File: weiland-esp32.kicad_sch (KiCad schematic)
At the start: 19 parts, among them J1 Conn_01x04_Pin, J2 Conn_01x05_Pin, J5 Conn_02x03_Odd_Even, U1 ESP32-WROOM-32E(8MB), U2 AMS1117-3.3_C347222, U3 GR6205-SOP-8, U4 MAX98357AEWL_T

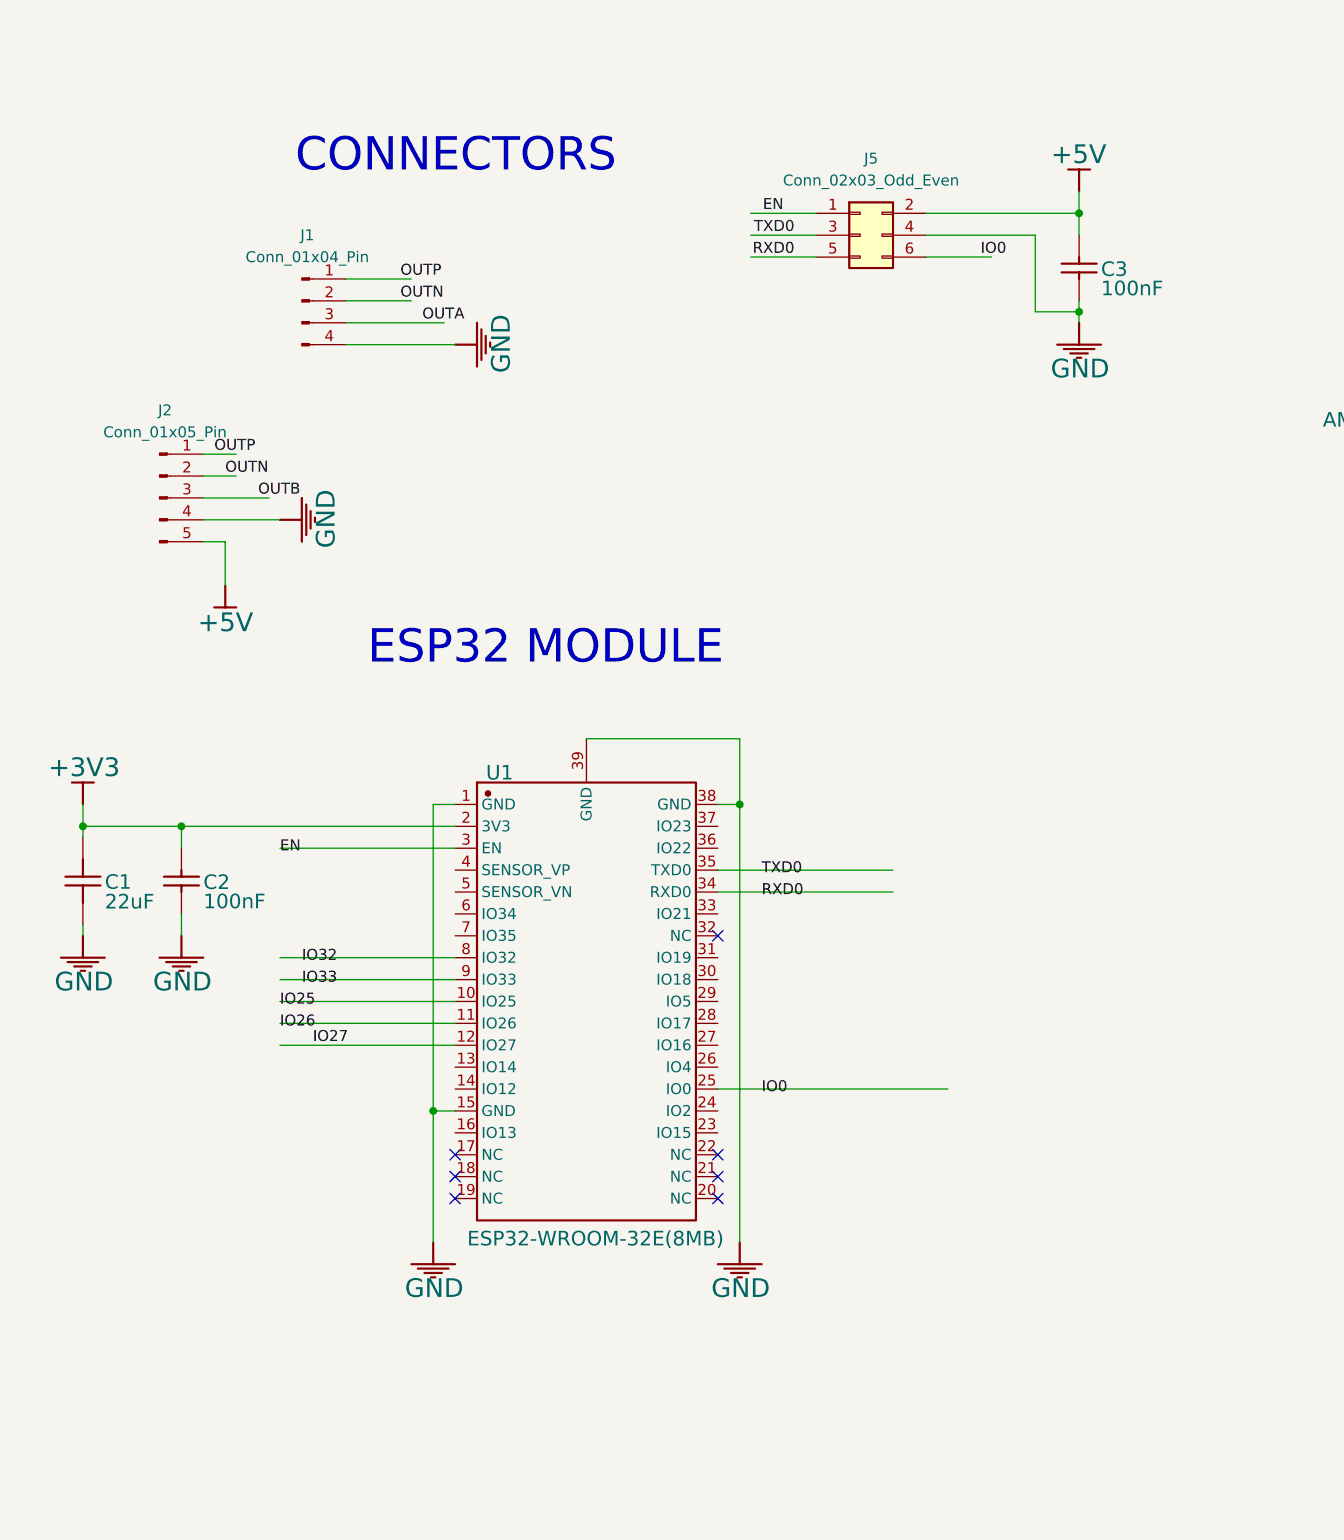
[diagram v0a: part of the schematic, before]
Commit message: jst connectors
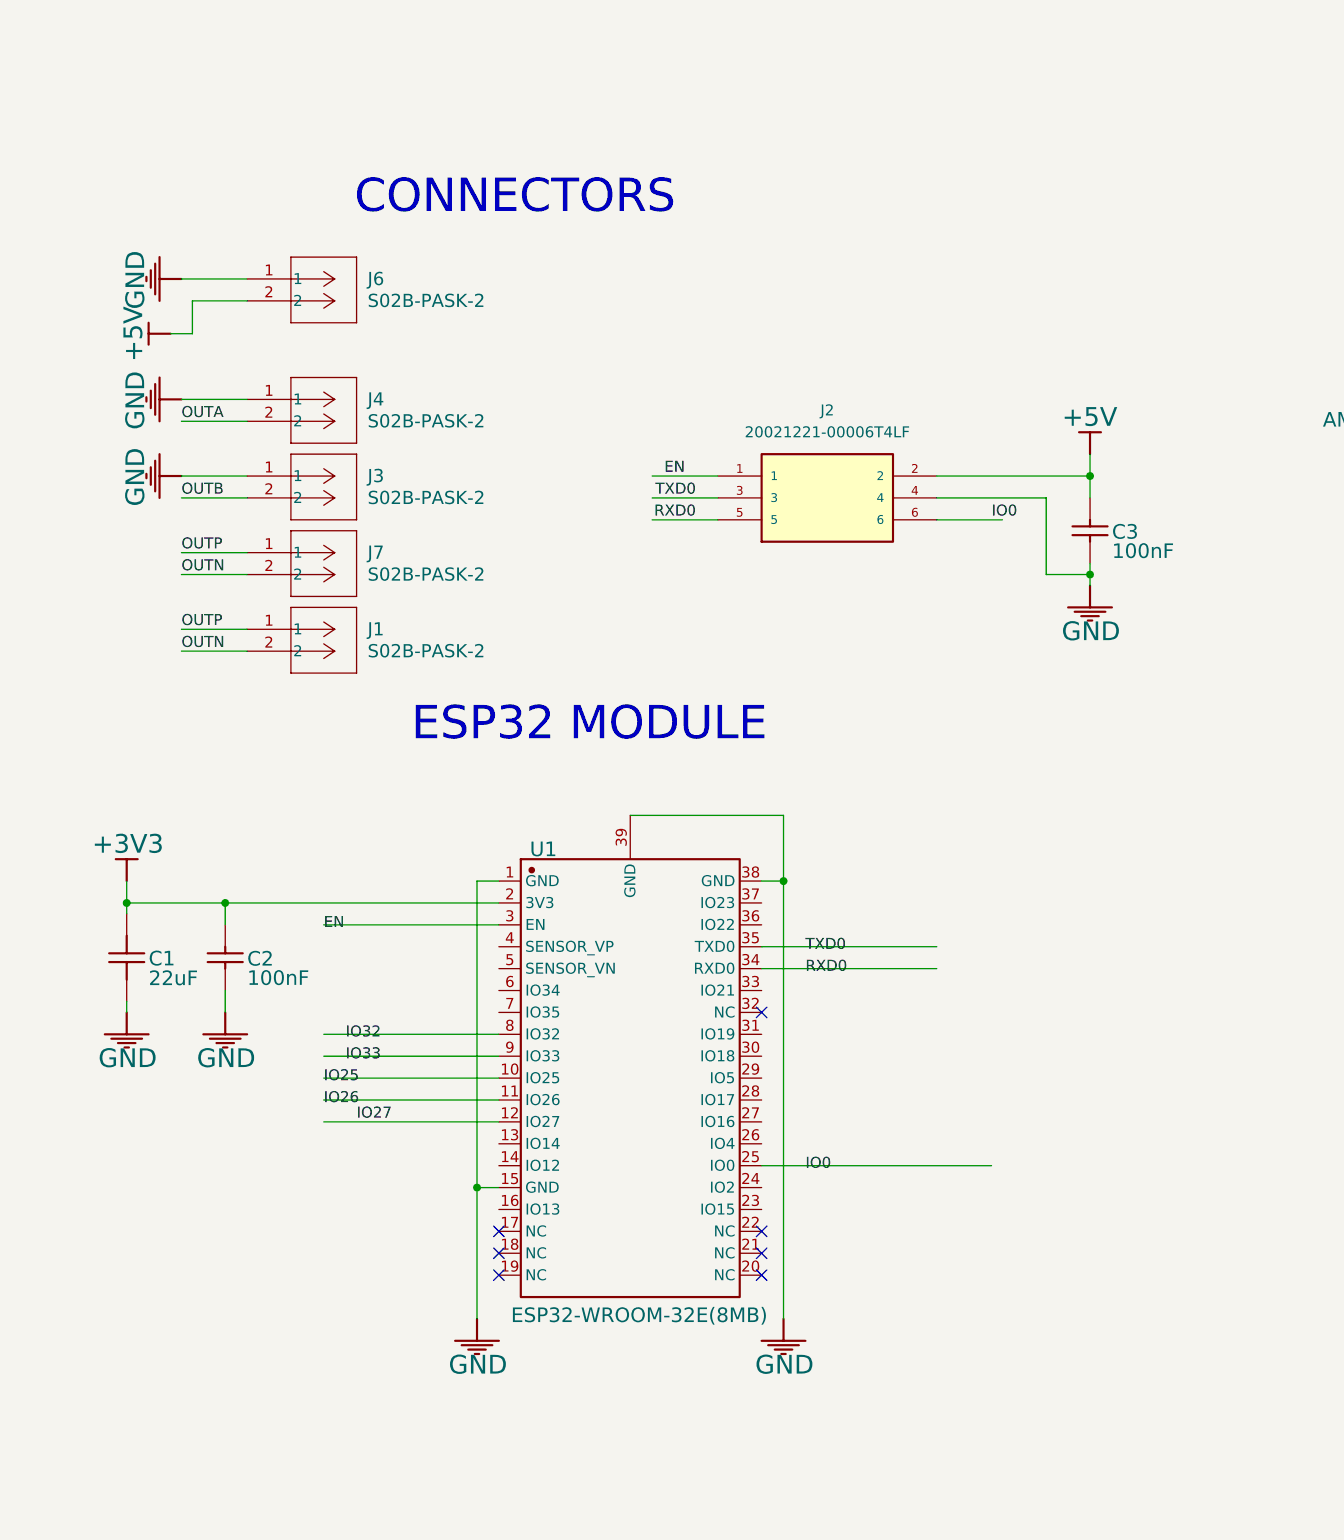
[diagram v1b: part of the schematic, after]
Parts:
- removed J1: Conn_01x04_Pin, Connector_Wire:SolderWire-0.75sqmm_1x04_P4.8mm_D1.25mm_OD2.3mm, symbol Connector:Conn_01x04_Pin
- removed J2: Conn_01x05_Pin, customlibrary:SolderWire-0.75sqmm_1x05_P4.8mm_D1.25mm_OD2.3mm, symbol Connector:Conn_01x05_Pin
- removed J5: Conn_02x03_Odd_Even, Connector_PinSocket_1.27mm:PinSocket_2x03_P1.27mm_Vertical_SMD, symbol Connector_Generic:Conn_02x03_Odd_Even
- added J1, J3, J4, J6, J7: S02B-PASK-2, footprints:CONN2_S02B-PASK-2_JST, symbol jst2pin:S02B-PASK-2
- added J2: 20021221-00006T4LF, dc3-6p:dc3-6p, symbol dc3-6p:20021221-00006T4LF
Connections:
- net +5V: now also J2.2, J6.2
- net EN: now also J2.1
- net GND: now also J2.4, J3.1, J4.1, J6.1
- net IO0: now also J2.6
- net OUTA: now also J4.2
- net OUTB: now also J3.2
- net OUTN: now also J1.2, J7.2
- net OUTP: now also J1.1, J7.1
- net RXD0: now also J2.5
- net TXD0: now also J2.3
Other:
- moved on the sheet: C1, C2, C3, U1
